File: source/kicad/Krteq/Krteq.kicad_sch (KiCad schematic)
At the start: 202 parts, among them J1 USB breakout board, J2 Pico test points, J3 OLED 128x32, SW1 GATERON Low Profile Switch Ho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, SW10 GATERON Low Profile Switch Ho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, SW11 GATERON Low Profile Switch Ho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, SW12 GATERON Low Profile Switch Ho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, SW13 GATERON Low Profile Switch Ho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, SW14 GATERON Low Profile Switch Ho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, SW15 GATERON Low Profile Switch Ho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, SW16 GATERON Low Profile Switch Ho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, SW17 GATERON Low Profile Switch Ho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, SW18 GATERON Low Profile Switch Ho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, SW19 GATERON Low Profile Switch Ho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, SW2 GATERON Low Profile Switch Ho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, SW20 GATERON Low Profile Switch Ho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, SW21 GATERON Low Profile Switch Ho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, SW22 GATERON Low Profile Switch Ho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, SW23 GATERON Low Profile Switch Ho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, SW24 GATERON Low Profile Switch Ho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, SW25 GATERON Low Profile Switch Ho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, SW26 GATERON Low Profile Switch Ho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, SW27 GATERON Low Profile Switch Ho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, SW28 GATERON Low Profile Switch Ho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, SW29 GATERON Low Profile Switch Ho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, SW3 GATERON Low Profile Switch Ho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, SW30 GATERON Low Profile Switch Ho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, SW31 GATERON Low Profile Switch Ho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, SW32 GATERON Low Profile Switch Ho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, SW33 GATERON Low Profile Switch Ho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, SW34 GATERON Low Profile Switch Ho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, SW35 GATERON Low Profile Switch Ho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, SW36 GATERON Low Profile Switch Ho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, SW37 GATERON Low Profile Switch Ho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, SW38 GATERON Low Profile Switch Ho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, SW39 GATERON Low Profile Switch Ho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, SW4 GATERON Low Profile Switch Ho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, SW40 GATERON Low Profile Switch Ho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, SW41 GATERON Low Profile Switch Ho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, SW42 GATERON Low Profile Switch Ho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, SW43 GATERON Low Profile Switch Ho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, SW44 GATERON Low Profile Switch Ho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, SW45 GATERON Low Profile Switch Ho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, SW46 GATERON Low Profile Switch Ho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, SW47 GATERON Low Profile Switch Ho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, SW48 GATERON Low Profile Switch Ho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, SW49 GATERON Low Profile Switch Ho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, SW5 GATERON Low Profile Switch Ho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, SW50 GATERON Low Profile Switch Ho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, SW51 GATERON Low Profile Switch Ho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, SW52 GATERON Low Profile Switch Ho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, SW53 GATERON Low Profile Switch Ho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, SW54 GATERON Low Profile Switch Ho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, SW55 GATERON Low Profile Switch Ho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, SW56 GATERON Low Profile Switch Ho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, SW57 GATERON Low Profile Switch Ho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, SW58 GATERON Low Profile Switch Ho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, SW59 GATERON Low Profile Switch Ho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, SW6 GATERON Low Profile Switch Ho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, SW60 GATERON Low Profile Switch Ho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, SW61 GATERON Low Profile Switch Ho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, SW7 GATERON Low Profile Switch Ho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, SW8 GATERON Low Profile Switch Ho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, SW9 GATERON Low Profile Switch Ho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, U71 LED Driver

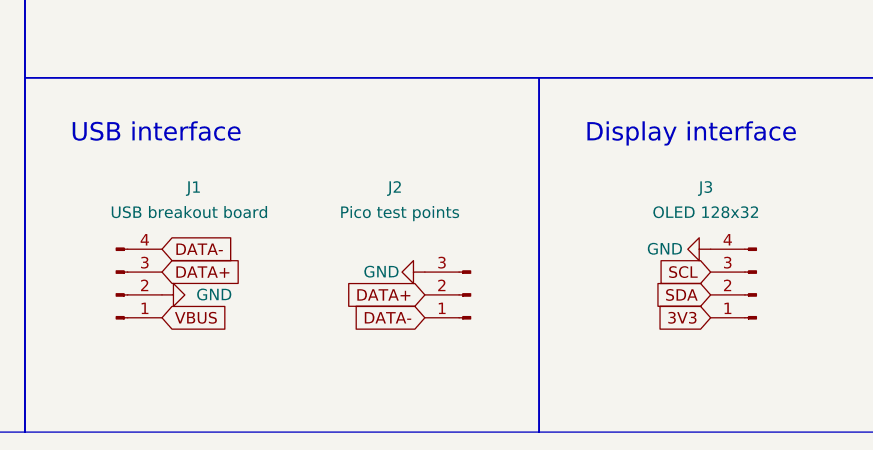
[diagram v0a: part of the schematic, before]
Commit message: update
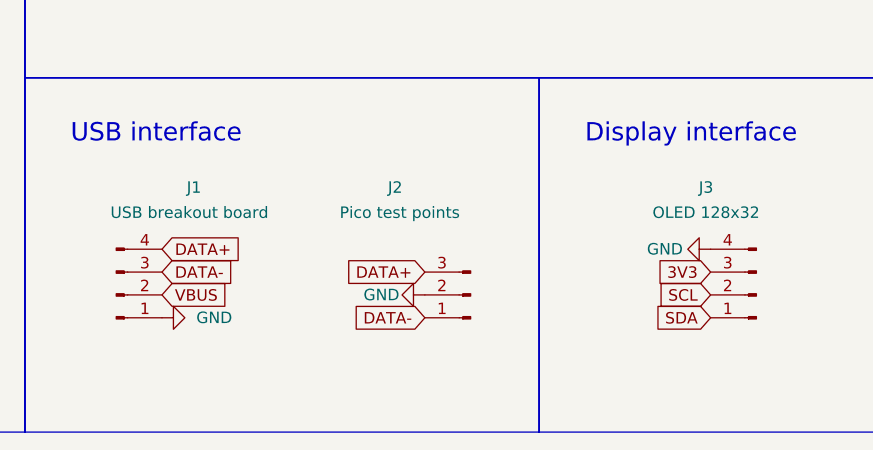
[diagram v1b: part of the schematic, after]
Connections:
- net 3V3: now also J3.3 (Pin_3); no longer J3.1 (Pin_1)
- net DATA+: now also J1.4 (Pin_4), J2.3 (Pin_3); no longer J1.3 (Pin_3), J2.2 (Pin_2)
- net DATA-: now also J1.3 (Pin_3); no longer J1.4 (Pin_4)
- net GND: now also J1.1 (Pin_1), J2.2 (Pin_2); no longer J1.2 (Pin_2), J2.3 (Pin_3)
- net SCL: now also J3.2 (Pin_2); no longer J3.3 (Pin_3)
- net SDA: now also J3.1 (Pin_1); no longer J3.2 (Pin_2)
- net VBUS: now also J1.2 (Pin_2); no longer J1.1 (Pin_1)
